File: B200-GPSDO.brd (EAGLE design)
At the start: 28.6 x 33.7 mm, 8 parts, among them U1 LEA-6T, U2 NC7SZ125, U3 NC7SZ125, U4 GPSDO

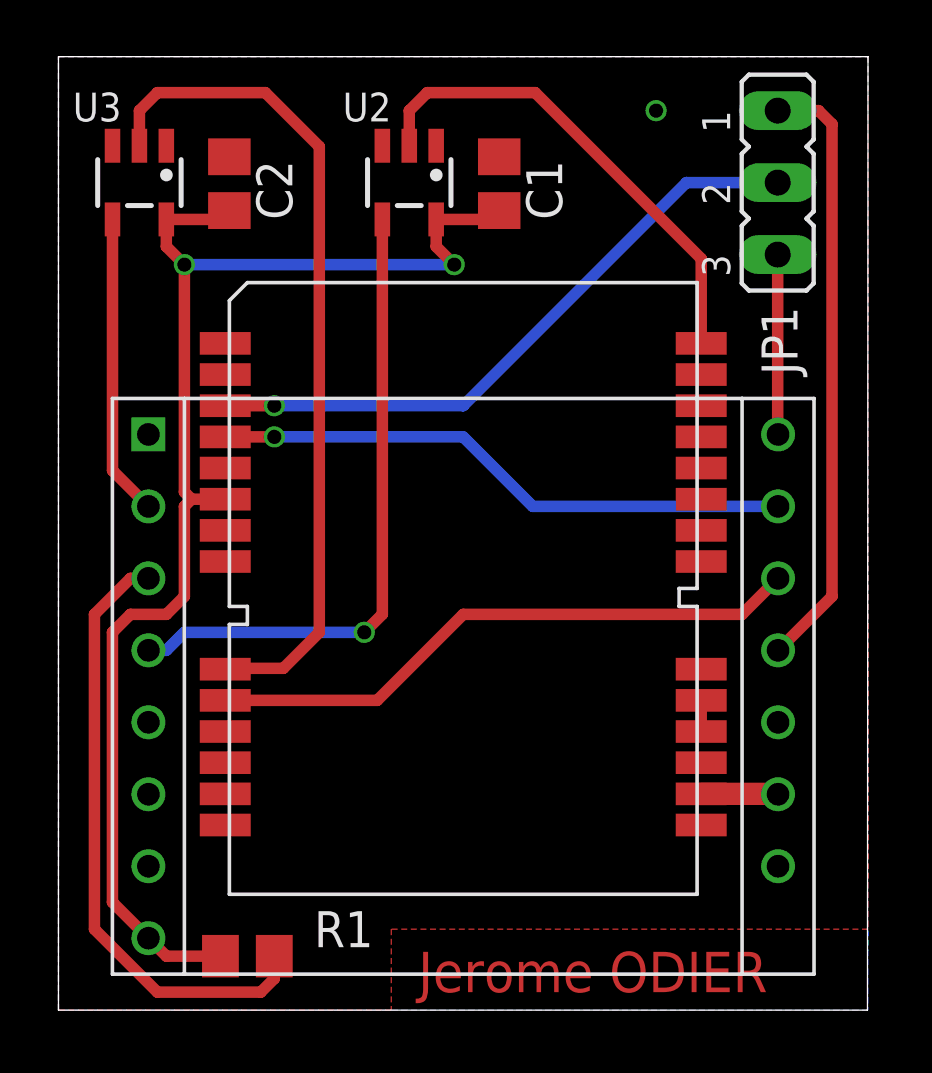
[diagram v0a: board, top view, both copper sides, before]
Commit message: update
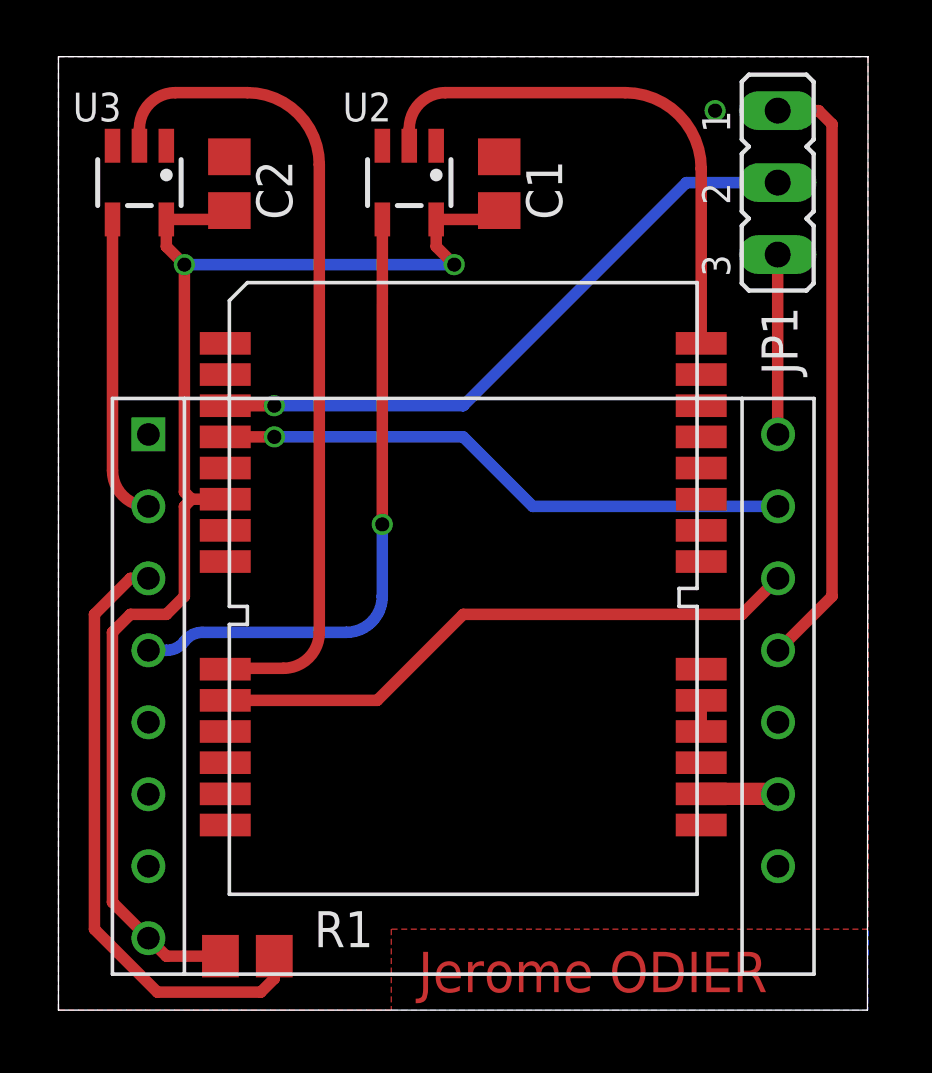
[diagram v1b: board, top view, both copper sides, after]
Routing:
- net N$4: track 17.2 -> 18.7 mm
- net N$3: track 29.6 -> 28.9 mm
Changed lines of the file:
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@@
 <setting verticaltext="up"/>
 </settings>
-<grid distance="0.025" unitdist="inch" unit="inch" style="lines" multiple="1" display="yes" altdistance="0.025" altunitdist="inch" altunit="inch"/>
+<grid distance="0.0125" unitdist="inch" unit="inch" style="lines" multiple="1" display="yes" altdistance="0.025" altunitdist="inch" altunit="inch"/>
 <layers>
 <layer number="1" name="Top" color="4" fill="1" visible="yes" active="yes"/>
@@
 <wire x1="2.8575" y1="2.54" x2="1.5875" y2="3.81" width="0.4064" layer="1"/>
 <wire x1="1.5875" y1="3.81" x2="1.5875" y2="13.335" width="0.4064" layer="1"/>
-<wire x1="1.5875" y1="13.335" x2="2.2225" y2="13.97" width="0.4064" layer="1"/>
 <wire x1="5.57" y1="18.0344" x2="4.3819" y2="18.0344" width="0.4064" layer="1"/>
 <wire x1="4.3819" y1="18.0344" x2="4.1275" y2="17.78" width="0.4064" layer="1"/>
@@
 <wire x1="3.49" y1="27.9099" x2="5.403" y2="27.9099" width="0.4064" layer="1"/>
 <wire x1="5.403" y1="27.9099" x2="5.715" y2="28.2219" width="0.4064" layer="1"/>
+<wire x1="1.5875" y1="13.335" x2="2.2225" y2="13.97" width="0.4064" layer="1"/>
 </signal>
 <signal name="RXD">
@@
 <contactref element="U3" pad="2"/>
 <contactref element="U1" pad="9"/>
-<wire x1="8.89" y1="30.48" x2="6.985" y2="32.385" width="0.4064" layer="1"/>
-<wire x1="6.985" y1="32.385" x2="3.175" y2="32.385" width="0.4064" layer="1"/>
-<wire x1="2.54" y1="30.5101" x2="2.54" y2="31.75" width="0.4064" layer="1"/>
-<wire x1="2.54" y1="31.75" x2="3.175" y2="32.385" width="0.4064" layer="1"/>
-<wire x1="8.89" y1="30.48" x2="8.89" y2="13.335" width="0.4064" layer="1"/>
-<wire x1="8.89" y1="13.335" x2="7.62" y2="12.065" width="0.4064" layer="1"/>
-<wire x1="7.62" y1="12.065" x2="5.6006" y2="12.065" width="0.4064" layer="1"/>
+<wire x1="8.89" y1="29.845" x2="8.89" y2="13.335" width="0.4064" layer="1"/>
 <wire x1="5.6006" y1="12.065" x2="5.57" y2="12.0344" width="0.4064" layer="1"/>
+<wire x1="5.6006" y1="12.065" x2="7.62" y2="12.065" width="0.4064" layer="1"/>
+<wire x1="3.81" y1="32.385" x2="6.35" y2="32.385" width="0.4064" layer="1"/>
+<wire x1="2.54" y1="30.5101" x2="2.54" y2="31.115" width="0.4064" layer="1"/>
+<wire x1="2.54" y1="31.115" x2="3.81" y2="32.385" width="0.4064" layer="1" curve="-90"/>
+<wire x1="6.35" y1="32.385" x2="8.89" y2="29.845" width="0.4064" layer="1" curve="-90"/>
+<wire x1="7.62" y1="12.065" x2="8.89" y2="13.335" width="0.4064" layer="1" curve="90"/>
 </signal>
 <signal name="N$4">
 <contactref element="U2" pad="2"/>
 <contactref element="U1" pad="28"/>
-<wire x1="12.065" y1="30.5101" x2="12.065" y2="31.75" width="0.4064" layer="1"/>
-<wire x1="12.065" y1="31.75" x2="12.7" y2="32.385" width="0.4064" layer="1"/>
-<wire x1="12.7" y1="32.385" x2="16.51" y2="32.385" width="0.4064" layer="1"/>
-<wire x1="16.51" y1="32.385" x2="22.37" y2="26.525" width="0.4064" layer="1"/>
-<wire x1="22.37" y1="23.5344" x2="22.37" y2="26.525" width="0.4064" layer="1"/>
+<wire x1="12.065" y1="30.5101" x2="12.065" y2="31.115" width="0.4064" layer="1"/>
+<wire x1="12.065" y1="31.115" x2="13.335" y2="32.385" width="0.4064" layer="1" curve="-90"/>
+<wire x1="22.37" y1="23.5344" x2="22.37" y2="29.7" width="0.4064" layer="1"/>
+<wire x1="19.685" y1="32.385" x2="13.335" y2="32.385" width="0.4064" layer="1"/>
+<wire x1="19.685" y1="32.385" x2="22.37" y2="29.7" width="0.4064" layer="1" curve="-90"/>
 </signal>
 <signal name="RF_IN">
@@
 <vertex x="-0.3175" y="0"/>
 </polygon>
-<via x="20.7772" y="31.75" extent="1-16" drill="0.5"/>
+<via x="22.86" y="31.75" extent="1-16" drill="0.5"/>
 <contactref element="U1" pad="11"/>
 </signal>
@@
 <contactref element="U2" pad="4"/>
 <contactref element="U4" pad="4"/>
-<wire x1="11.115" y1="27.9099" x2="11.115" y2="13.9725" width="0.4064" layer="1"/>
-<via x="10.4775" y="13.335" extent="1-16" drill="0.5"/>
-<wire x1="11.115" y1="13.9725" x2="10.4775" y2="13.335" width="0.4064" layer="1"/>
-<wire x1="10.4775" y1="13.335" x2="4.1275" y2="13.335" width="0.4064" layer="16"/>
-<wire x1="4.1275" y1="13.335" x2="3.4925" y2="12.7" width="0.4064" layer="16"/>
+<via x="11.1125" y="17.145" extent="1-16" drill="0.5"/>
 <wire x1="3.4925" y1="12.7" x2="2.8575" y2="12.7" width="0.4064" layer="16"/>
+<wire x1="4.7625" y1="13.335" x2="9.8425" y2="13.335" width="0.4064" layer="16"/>
+<wire x1="3.4925" y1="12.7" x2="4.1275" y2="13.0175" width="0.4064" layer="16" curve="53.130102"/>
+<wire x1="4.1275" y1="13.0175" x2="4.7625" y2="13.335" width="0.4064" layer="16" curve="-53.130102"/>
+<wire x1="11.115" y1="27.9099" x2="11.1125" y2="17.145" width="0.4064" layer="1"/>
+<wire x1="11.1125" y1="17.145" x2="11.1125" y2="14.605" width="0.4064" layer="16"/>
+<wire x1="11.1125" y1="14.605" x2="9.8425" y2="13.335" width="0.4064" layer="16" curve="-90"/>
 </signal>
 <signal name="10MHZ">
@@
 <contactref element="U4" pad="2"/>
 <wire x1="1.59" y1="27.9099" x2="1.59" y2="19.0475" width="0.4064" layer="1"/>
-<wire x1="1.59" y1="19.0475" x2="2.8575" y2="17.78" width="0.4064" layer="1"/>
+<wire x1="1.59" y1="19.0475" x2="2.8575" y2="17.78" width="0.4064" layer="1" curve="90"/>
 </signal>
 <signal name="!RESET">
